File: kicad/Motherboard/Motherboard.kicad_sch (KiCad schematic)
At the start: 52 parts, among them J1 USB_C_Receptacle_USB2.0, J2 Conn_01x16_Pin, J3 Conn_01x16_Pin, J4 Conn_01x16_Pin, J5 Conn_01x02_Pin, J6 Conn_01x04_Pin, J7 Conn_01x04_Pin, J8 Conn_01x16_Pin, Q1 DMN3404L, SW1 Reset, SW2 Boot, U1 ESP32-S2-SOLO, U2 LD1117S33TR_SOT223, U3 CD74HC4067M, U4 CD74HC4067M, U5 CD74HC4067M, U6 CD74HC4067M, U7 TMC2208-LA, U8 TMC2208-LA, U9 LM2575-5.0BT

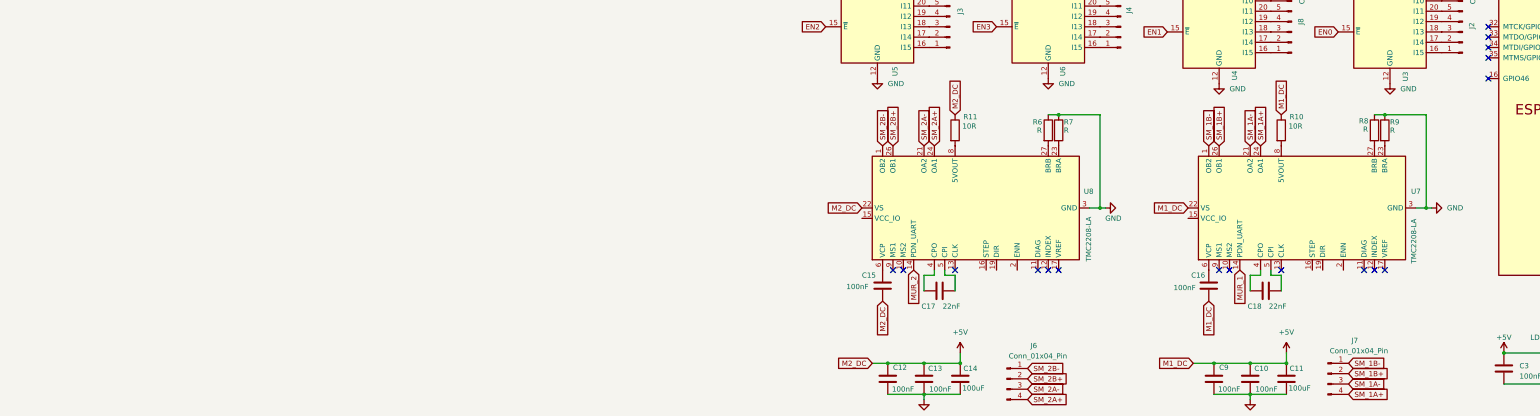
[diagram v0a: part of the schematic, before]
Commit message: tmcs done
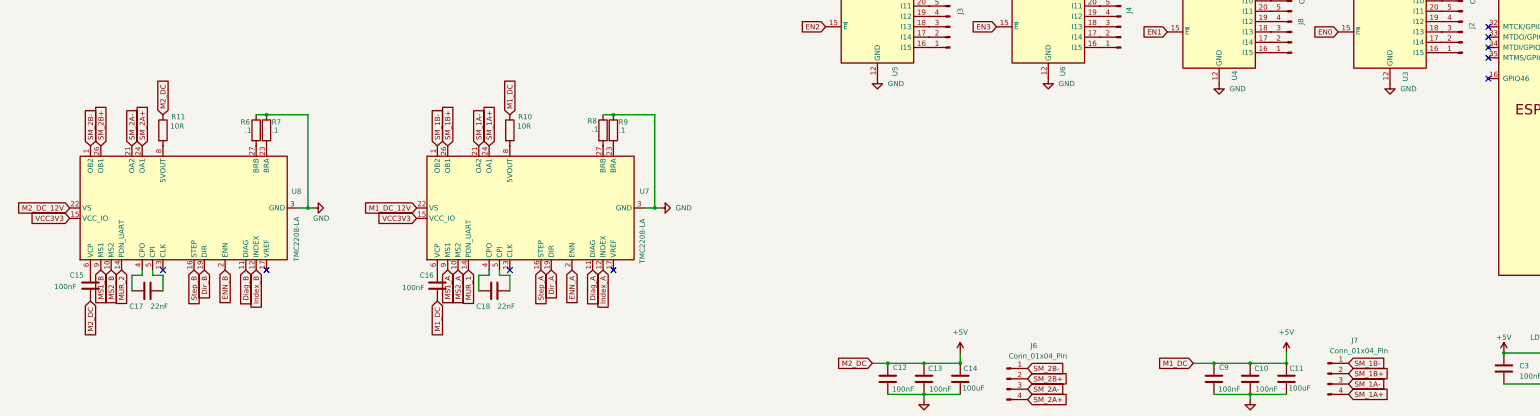
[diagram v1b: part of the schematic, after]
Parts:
- R6, R7, R8, R9: value R -> .1
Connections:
- net +5V: no longer U7.22 (VS), U7.28 (VS), U8.22 (VS), U8.28 (VS)
- net MS2_A: now reaches U7.10 (MS2)
- net Diag_A: now reaches U7.11 (DIAG)
- net Index_A: now reaches U7.12 (INDEX)
- net VCC3V3: now reaches U7.15 (VCC_IO)
- net VCC3V3: now also U8.15 (VCC_IO)
- net Step_A: now reaches U7.16 (STEP)
- net Dir_A: now reaches U7.19 (DIR)
- net ENN_A: now reaches U7.2 (ENN)
- net MS1_A: now reaches U7.9 (MS1)
- net MS2_B: now reaches U8.10 (MS2)
- net Diag_B: now reaches U8.11 (DIAG)
- net Index_B: now reaches U8.12 (INDEX)
- net Step_B: now reaches U8.16 (STEP)
- net Dir_B: now reaches U8.19 (DIR)
- net ENN_B: now reaches U8.2 (ENN)
- net MS1_B: now reaches U8.9 (MS1)
- new net M1_DC_12V: U7.22 (VS), U7.28 (VS)
- new net M2_DC_12V: U8.22 (VS), U8.28 (VS)
- no-connect marks 29 -> 21
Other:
- moved on the sheet: C15, C16, C17, C18, R10, R11, R6, R7, R8, R9, U7, U8

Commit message: penultimate schematic
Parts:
- removed R10, R11: 10R, symbol Device:R
- added C19: 2.2uF, Capacitor_SMD:C_0603_1608Metric_Pad1.08x0.95mm_HandSolder, symbol Device:C
- added C20, C21, C22, C23, C24: 22uF, Capacitor_SMD:C_0805_2012Metric_Pad1.18x1.45mm_HandSolder, symbol Device:C
- C10, C13, C9: value 100nF -> 22uF; footprint (none) -> Capacitor_SMD:C_0805_2012Metric_Pad1.18x1.45mm_HandSolder
- C11, C14: value 100uF -> 22uF; footprint (none) -> Capacitor_SMD:C_0805_2012Metric_Pad1.18x1.45mm_HandSolder
- C12: footprint (none) -> Capacitor_SMD:C_0402_1005Metric_Pad0.74x0.62mm_HandSolder
- C15: value 100nF -> 2.2uF; footprint (none) -> Capacitor_SMD:C_0603_1608Metric_Pad1.08x0.95mm_HandSolder
- C16: value 100nF -> 22nF; footprint (none) -> Capacitor_SMD:C_0201_0603Metric_Pad0.64x0.40mm_HandSolder
- C17: footprint (none) -> Capacitor_SMD:C_0201_0603Metric_Pad0.64x0.40mm_HandSolder
- C18: value 22nF -> 100nF; footprint (none) -> Capacitor_SMD:C_0402_1005Metric_Pad0.74x0.62mm_HandSolder
- D1, D2: footprint (none) -> Diode_THT:D_DO-41_SOD81_P5.08mm_Vertical_AnodeUp
- J2, J3, J4, J8: footprint (none) -> Connector_PinHeader_1.27mm:PinHeader_1x16_P1.27mm_Horizontal
- J5: footprint (none) -> Connector_PinHeader_1.27mm:PinHeader_1x02_P1.27mm_Horizontal
- J6, J7: footprint (none) -> Connector_PinHeader_1.27mm:PinHeader_1x04_P1.27mm_Horizontal
- L1: footprint (none) -> Inductor_SMD:L_1008_2520Metric_Pad1.43x2.20mm_HandSolder
- R6, R7, R8, R9: footprint (none) -> Resistor_SMD:R_0805_2012Metric_Pad1.20x1.40mm_HandSolder
- U1: footprint PCM_Espressif:ESP32-S2-SOLO -> RF_Module:ESP32-S2-MINI-1
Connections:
- net Dir_A is gone; now on net DIR_2: U7.19 (DIR)
- net Dir_B is gone; now on net DIR_1: U8.19 (DIR)
- net ENN_A is gone; now on net ENN_2: U7.2 (ENN)
- net ENN_B is gone; now on net ENN_1: U8.2 (ENN)
- net M1_DC_12V is gone; now on net +12V: U7.22 (VS), U7.28 (VS)
- net M2_DC_12V is gone; now on net +12V: U8.22 (VS), U8.28 (VS)
- net MUR_1 is gone; now on net UART_2: U7.14 (PDN_UART)
- net MUR_2 is gone; now on net UART_1: U8.14 (PDN_UART)
- net Step_A is gone; now on net STEP_2: U7.16 (STEP)
- net Step_B is gone; now on net STEP_1: U8.16 (STEP)
- net VCC3V3 is gone; now on net +3.3V: U7.15 (VCC_IO), U8.15 (VCC_IO)
- net +12V: now also C10.1, C11.1, C12.1, C13.2, C14.2, C18.1, C9.1, C20.1, C21.2, C22.1, C23.2, C24.1
- net +5V: no longer C10.1, C11.1, C12.1, C13.1, C14.1, C15.2, C16.2, C9.1
- net GND: now also C13.1, C14.1, C15.1, C19.1, C20.2, C21.1, C22.2, C23.1, C24.2; no longer C12.2, C13.2, C14.2
- net MAGCT: now also U1.29 (SPIIO7/GPIO36/FSPICLK); no longer U1.26 (GPIO45)
- net at C16.1: now also U7.4 (CPO); no longer U7.6 (VCP)
- net at U7.5 (CPI): now also C16.2; no longer C18.2
- net 5VOUT_2: now reaches U7.8 (5VOUT)
- net 5VOUT_2: now also C19.2
- net STEP_1: now reaches U1.10 (GPIO17/U1TXD/ADC2_CH6/DAC_1)
- net UART_1: now reaches U1.11 (GPIO18/U1RXD/ADC2_CH7/DAC_2/CLK_OUT3)
- net ENN_1: now reaches U1.21 (GPIO13/TOUCH13/ADC2_CH2/FSPIQ/FSPIIO7)
- net DIR_1: now reaches U1.22 (GPIO14/TOUCH14/ADC2_CH3/FSPIWP/FSPIDQS)
- net ENN_2: now reaches U1.23 (GPIO21)
- net DIR_2: now reaches U1.24 (SPIIO4/GPIO33/FSPIHD)
- net STEP_2: now reaches U1.25 (SPIIO5/GPIO34/FSPICS0)
- net UART_2: now reaches U1.28 (SPIIO6/GPIO35/FSPID)
- net VCP_1: now reaches U8.6 (VCP)
- net VCP_1: now also C12.2; no longer C15.1
- net 5VOUT_1: now reaches U8.8 (5VOUT)
- net 5VOUT_1: now also C15.2
- net Diag_A: no longer names the net of U7.11 (DIAG)
- net Diag_B: no longer names the net of U8.11 (DIAG)
- net Index_A: no longer names the net of U7.12 (INDEX)
- net Index_B: no longer names the net of U8.12 (INDEX)
- net MS1_A: no longer names the net of U7.9 (MS1)
- net MS1_B: no longer names the net of U8.9 (MS1)
- net MS2_A: no longer names the net of U7.10 (MS2)
- net MS2_B: no longer names the net of U8.10 (MS2)
- net SM_1A+ renamed Motor1_2
- net SM_1A- renamed Motor2_2
- net SM_1B+ renamed Motor3_2
- net SM_1B- renamed Motor4_2
- net SM_2A+ renamed Motor1_1
- net SM_2A- renamed Motor2_1
- net SM_2B+ renamed Motor3_1
- net SM_2B- renamed Motor4_1
- new net VCP_2: C18.2, U7.6 (VCP)
- no-connect marks 21 -> 28
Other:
- moved on the sheet: C10, C11, C17, C3, C6, C7, C8, C9, D1, D2, J5, J6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

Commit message: updated layout
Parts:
- C1, C12, C18, C3, C4, C5: footprint Capacitor_SMD:C_0402_1005Metric_Pad0.74x0.62mm_HandSolder -> Capacitor_SMD:C_0805_2012Metric_Pad1.18x1.45mm_HandSolder
- C15, C19, C2: footprint Capacitor_SMD:C_0603_1608Metric_Pad1.08x0.95mm_HandSolder -> Capacitor_SMD:C_0805_2012Metric_Pad1.18x1.45mm_HandSolder
- C16, C17: footprint Capacitor_SMD:C_0201_0603Metric_Pad0.64x0.40mm_HandSolder -> Capacitor_SMD:C_0805_2012Metric_Pad1.18x1.45mm_HandSolder
- C7: footprint Capacitor_SMD:C_1206_3216Metric_Pad1.33x1.80mm_HandSolder -> Capacitor_SMD:C_0805_2012Metric_Pad1.18x1.45mm_HandSolder
- J1: footprint Button_Switch_SMD:SW_Push_SPST_NO_Alps_SKRK -> Connector_USB:USB_C_Receptacle_HRO_TYPE-C-31-M-12
- R1, R2, R3, R4, R5: footprint Resistor_SMD:R_0402_1005Metric_Pad0.72x0.64mm_HandSolder -> Resistor_SMD:R_0805_2012Metric_Pad1.20x1.40mm_HandSolder
- U1: footprint RF_Module:ESP32-S2-MINI-1 -> Espressif:ESP32-S2-SOLO
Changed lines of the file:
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@@
 			)
 		)
-		(property "Footprint" "Capacitor_SMD:C_0201_0603Metric_Pad0.64x0.40mm_HandSolder"
+		(property "Footprint" "Capacitor_SMD:C_0805_2012Metric_Pad1.18x1.45mm_HandSolder"
 			(at 36.5252 101.6 0)
 			(effects
@@
 			)
 		)
-		(property "Footprint" "Capacitor_SMD:C_0603_1608Metric_Pad1.08x0.95mm_HandSolder"
+		(property "Footprint" "Capacitor_SMD:C_0805_2012Metric_Pad1.18x1.45mm_HandSolder"
 			(at 229.5652 31.75 0)
 			(effects
@@
 			)
 		)
-		(property "Footprint" "Resistor_SMD:R_0402_1005Metric_Pad0.72x0.64mm_HandSolder"
+		(property "Footprint" "Resistor_SMD:R_0805_2012Metric_Pad1.20x1.40mm_HandSolder"
 			(at 142.24 187.452 90)
 			(effects
@@
 			)
 		)
-		(property "Footprint" "Capacitor_SMD:C_0402_1005Metric_Pad0.74x0.62mm_HandSolder"
+		(property "Footprint" "Capacitor_SMD:C_0805_2012Metric_Pad1.18x1.45mm_HandSolder"
 			(at 192.7352 27.94 0)
 			(effects
@@
 			)
 		)
-		(property "Footprint" "Capacitor_SMD:C_0402_1005Metric_Pad0.74x0.62mm_HandSolder"
+		(property "Footprint" "Capacitor_SMD:C_0805_2012Metric_Pad1.18x1.45mm_HandSolder"
 			(at 106.68 154.6352 0)
 			(effects
@@
 			)
 		)
-		(property "Footprint" "Capacitor_SMD:C_0402_1005Metric_Pad0.74x0.62mm_HandSolder"
+		(property "Footprint" "Capacitor_SMD:C_0805_2012Metric_Pad1.18x1.45mm_HandSolder"
 			(at 261.62 21.2852 0)
 			(effects
@@
 			)
 		)
-		(property "Footprint" "Capacitor_SMD:C_1206_3216Metric_Pad1.33x1.80mm_HandSolder"
+		(property "Footprint" "Capacitor_SMD:C_0805_2012Metric_Pad1.18x1.45mm_HandSolder"
 			(at 41.6052 182.88 0)
 			(effects
@@
 			)
 		)
-		(property "Footprint" "RF_Module:ESP32-S2-MINI-1"
+		(property "Footprint" "Espressif:ESP32-S2-SOLO"
 			(at 228.6 133.35 0)
 			(effects
@@
 			)
 		)
-		(property "Footprint" "Resistor_SMD:R_0402_1005Metric_Pad0.72x0.64mm_HandSolder"
+		(property "Footprint" "Resistor_SMD:R_0805_2012Metric_Pad1.20x1.40mm_HandSolder"
 			(at 140.208 185.42 90)
 			(effects
@@
 			)
 		)
-		(property "Footprint" "Capacitor_SMD:C_0402_1005Metric_Pad0.74x0.62mm_HandSolder"
+		(property "Footprint" "Capacitor_SMD:C_0805_2012Metric_Pad1.18x1.45mm_HandSolder"
 			(at 183.8452 146.05 0)
 			(effects
@@
 			)
 		)
-		(property "Footprint" "Resistor_SMD:R_0402_1005Metric_Pad0.72x0.64mm_HandSolder"
+		(property "Footprint" "Resistor_SMD:R_0805_2012Metric_Pad1.20x1.40mm_HandSolder"
 			(at 255.778 158.75 90)
 			(effects
@@
 			)
 		)
-		(property "Footprint" "Capacitor_SMD:C_0603_1608Metric_Pad1.08x0.95mm_HandSolder"
+		(property "Footprint" "Capacitor_SMD:C_0805_2012Metric_Pad1.18x1.45mm_HandSolder"
 			(at 45.72 153.3652 0)
 			(effects
@@
 			)
 		)
-		(property "Footprint" "Resistor_SMD:R_0402_1005Metric_Pad0.72x0.64mm_HandSolder"
+		(property "Footprint" "Resistor_SMD:R_0805_2012Metric_Pad1.20x1.40mm_HandSolder"
 			(at 207.01 31.242 90)
 			(effects
@@
 			)
 		)
-		(property "Footprint" "Capacitor_SMD:C_0402_1005Metric_Pad0.74x0.62mm_HandSolder"
+		(property "Footprint" "Capacitor_SMD:C_0805_2012Metric_Pad1.18x1.45mm_HandSolder"
 			(at 31.75 155.9052 0)
 			(effects
@@
 			)
 		)
-		(property "Footprint" "Capacitor_SMD:C_0603_1608Metric_Pad1.08x0.95mm_HandSolder"
+		(property "Footprint" "Capacitor_SMD:C_0805_2012Metric_Pad1.18x1.45mm_HandSolder"
 			(at 120.65 152.0952 0)
 			(effects
@@
 			)
 		)
-		(property "Footprint" "Capacitor_SMD:C_0201_0603Metric_Pad0.64x0.40mm_HandSolder"
+		(property "Footprint" "Capacitor_SMD:C_0805_2012Metric_Pad1.18x1.45mm_HandSolder"
 			(at 110.1852 101.6 0)
 			(effects
@@
 			)
 		)
-		(property "Footprint" "Capacitor_SMD:C_0402_1005Metric_Pad0.74x0.62mm_HandSolder"
+		(property "Footprint" "Capacitor_SMD:C_0805_2012Metric_Pad1.18x1.45mm_HandSolder"
 			(at 242.2652 31.75 0)
 			(effects
@@
 			)
 		)
-		(property "Footprint" "Resistor_SMD:R_0402_1005Metric_Pad0.72x0.64mm_HandSolder"
+		(property "Footprint" "Resistor_SMD:R_0805_2012Metric_Pad1.20x1.40mm_HandSolder"
 			(at 259.842 158.75 90)
 			(effects
@@
 			)
 		)
-		(property "Footprint" "Button_Switch_SMD:SW_Push_SPST_NO_Alps_SKRK"
+		(property "Footprint" "Connector_USB:USB_C_Receptacle_HRO_TYPE-C-31-M-12"
 			(at 251.46 140.97 0)
 			(effects

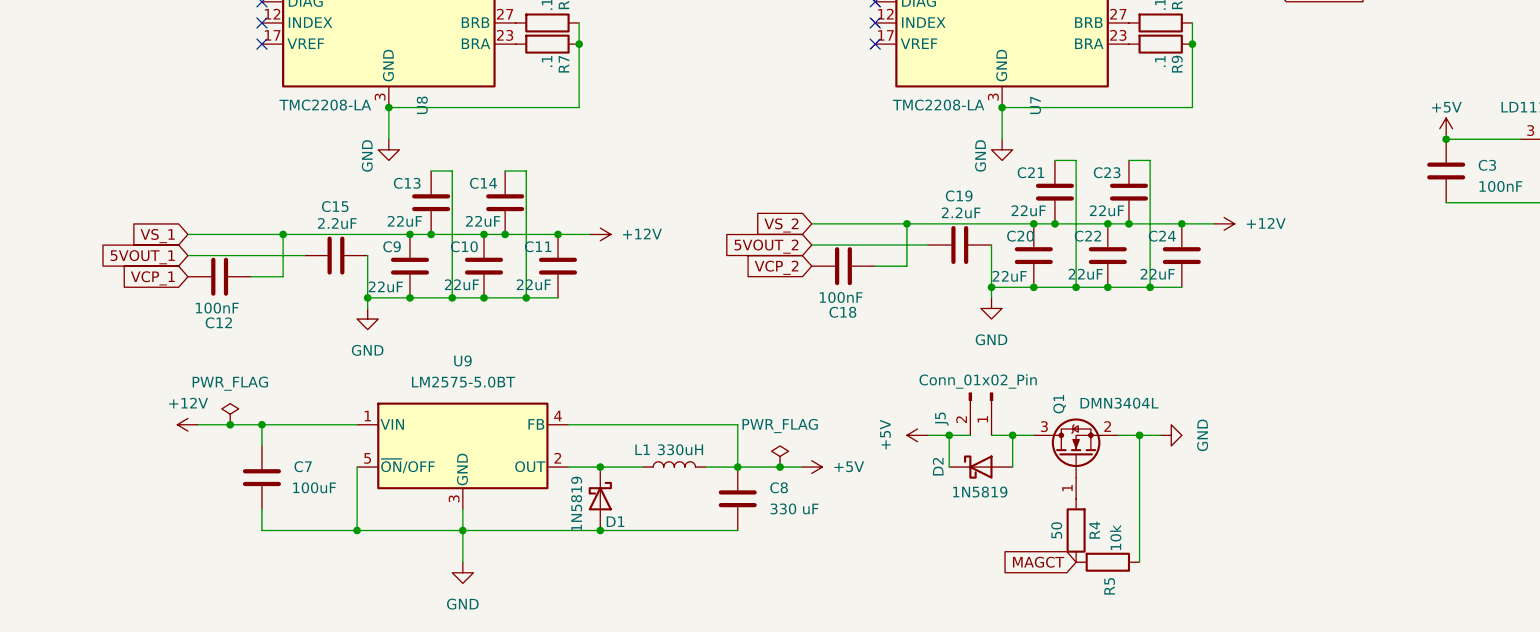
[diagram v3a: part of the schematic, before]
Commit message: updated schematic
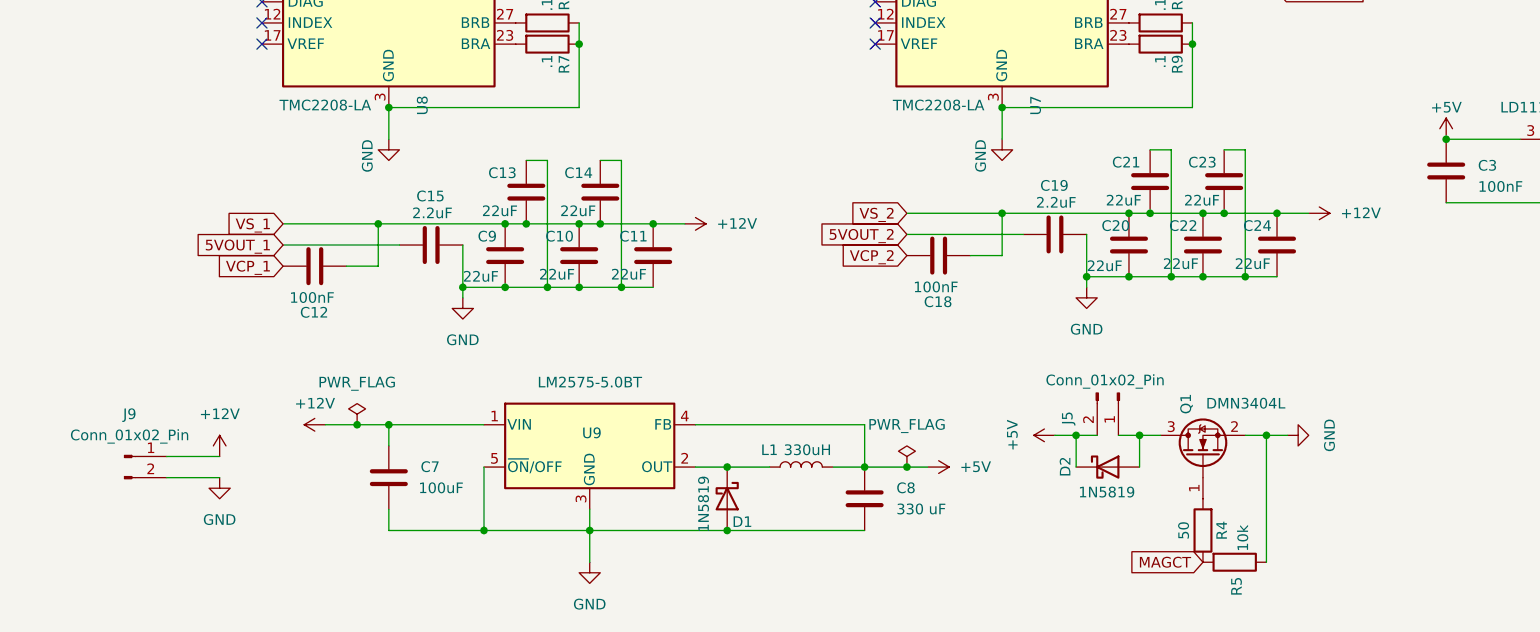
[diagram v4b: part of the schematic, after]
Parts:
- added J9: Conn_01x02_Pin, Connector_PinHeader_1.27mm:PinHeader_1x02_P1.27mm_Vertical, symbol Connector:Conn_01x02_Pin
- J2, J3, J4, J8: footprint Connector_PinHeader_1.27mm:PinHeader_1x16_P1.27mm_Horizontal -> Connector_PinHeader_1.27mm:PinHeader_1x16_P1.27mm_Vertical
- J5: footprint Connector_PinHeader_1.27mm:PinHeader_1x02_P1.27mm_Horizontal -> Connector_PinHeader_1.27mm:PinHeader_1x02_P1.27mm_Vertical
- J6, J7: footprint Connector_PinHeader_1.27mm:PinHeader_1x04_P1.27mm_Horizontal -> Connector_PinHeader_1.27mm:PinHeader_1x04_P1.27mm_Vertical
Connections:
- net +12V: now also J9.1 (Pin_1)
- net GND: now also J9.2 (Pin_2)
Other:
- moved on the sheet: C10, C11, C12, C13, C14, C15, C18, C19, C20, C21, C22, C23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

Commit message: bet
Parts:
- J2, J3, J4, J8: footprint Connector_PinHeader_1.27mm:PinHeader_1x16_P1.27mm_Vertical -> Connector_PinHeader_2.54mm:PinHeader_1x16_P2.54mm_Vertical
- J5, J9: footprint Connector_PinHeader_1.27mm:PinHeader_1x02_P1.27mm_Vertical -> Connector_PinHeader_2.54mm:PinHeader_1x02_P2.54mm_Vertical
- J6, J7: footprint Connector_PinHeader_1.27mm:PinHeader_1x04_P1.27mm_Vertical -> Connector_PinHeader_2.54mm:PinHeader_1x04_P2.54mm_Vertical
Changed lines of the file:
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@@
 			)
 		)
-		(property "Footprint" "Connector_PinHeader_1.27mm:PinHeader_1x16_P1.27mm_Vertical"
+		(property "Footprint" "Connector_PinHeader_2.54mm:PinHeader_1x16_P2.54mm_Vertical"
 			(at 176.53 48.26 0)
 			(effects
@@
 			)
 		)
-		(property "Footprint" "Connector_PinHeader_1.27mm:PinHeader_1x16_P1.27mm_Vertical"
+		(property "Footprint" "Connector_PinHeader_2.54mm:PinHeader_1x16_P2.54mm_Vertical"
 			(at 134.62 48.26 0)
 			(effects
@@
 			)
 		)
-		(property "Footprint" "Connector_PinHeader_1.27mm:PinHeader_1x16_P1.27mm_Vertical"
+		(property "Footprint" "Connector_PinHeader_2.54mm:PinHeader_1x16_P2.54mm_Vertical"
 			(at 92.71 46.99 0)
 			(effects
@@
 			)
 		)
-		(property "Footprint" "Connector_PinHeader_1.27mm:PinHeader_1x16_P1.27mm_Vertical"
+		(property "Footprint" "Connector_PinHeader_2.54mm:PinHeader_1x16_P2.54mm_Vertical"
 			(at 50.8 46.99 0)
 			(effects
@@
 			)
 		)
-		(property "Footprint" "Connector_PinHeader_1.27mm:PinHeader_1x04_P1.27mm_Vertical"
+		(property "Footprint" "Connector_PinHeader_2.54mm:PinHeader_1x04_P2.54mm_Vertical"
 			(at 82.55 114.3 0)
 			(effects
@@
 			)
 		)
-		(property "Footprint" "Connector_PinHeader_1.27mm:PinHeader_1x02_P1.27mm_Vertical"
+		(property "Footprint" "Connector_PinHeader_2.54mm:PinHeader_1x02_P2.54mm_Vertical"
 			(at 143.51 168.91 0)
 			(effects
@@
 			)
 		)
-		(property "Footprint" "Connector_PinHeader_1.27mm:PinHeader_1x02_P1.27mm_Vertical"
+		(property "Footprint" "Connector_PinHeader_2.54mm:PinHeader_1x02_P2.54mm_Vertical"
 			(at 24.13 176.53 0)
 			(effects
@@
 			)
 		)
-		(property "Footprint" "Connector_PinHeader_1.27mm:PinHeader_1x04_P1.27mm_Vertical"
+		(property "Footprint" "Connector_PinHeader_2.54mm:PinHeader_1x04_P2.54mm_Vertical"
 			(at 157.48 115.57 0)
 			(effects
